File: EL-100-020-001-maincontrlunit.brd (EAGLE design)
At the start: 68 x 86 mm, 13 parts, among them T1 WS-TST-90°, U19 ABS10-32.768KHZ-7-T, U8 MCP7940N-I/SN, U9 PMEG2005ET, X1 944-12-46-00, X2 944-12-46-00

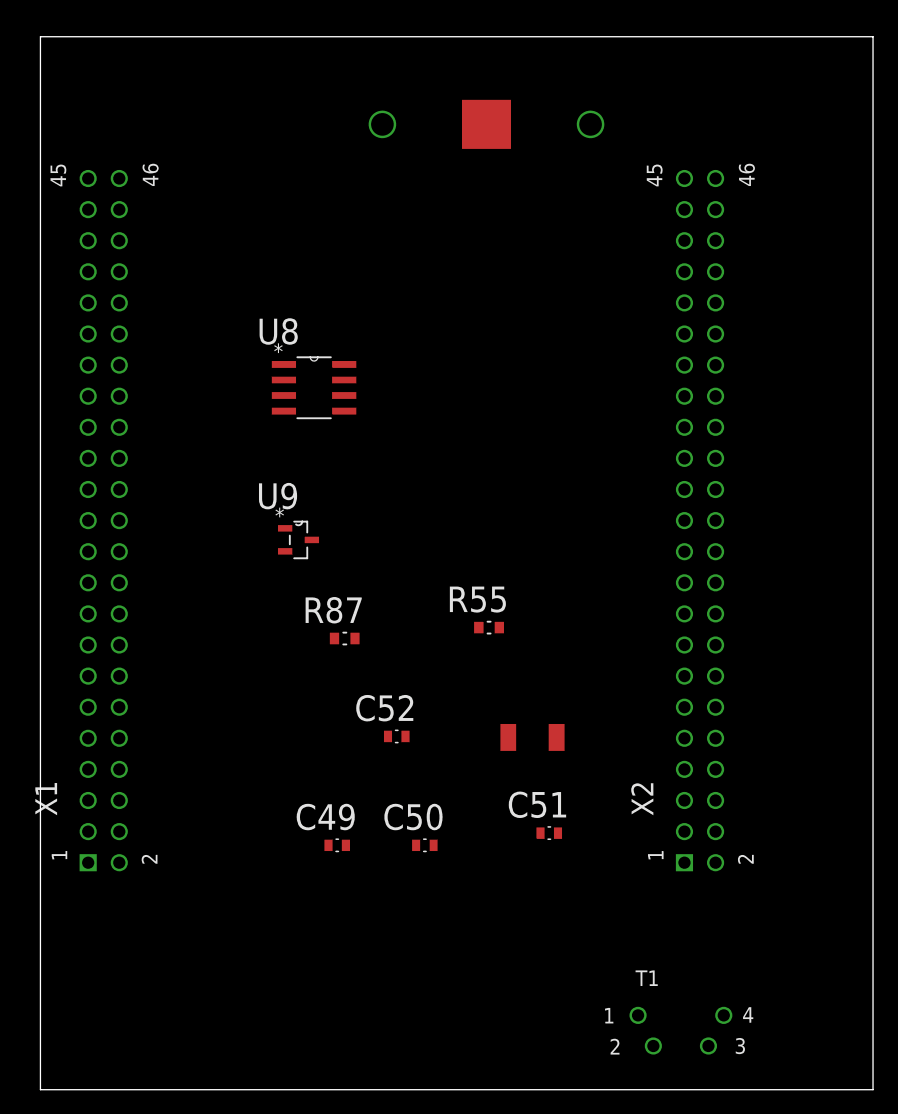
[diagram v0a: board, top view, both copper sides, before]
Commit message: update layout
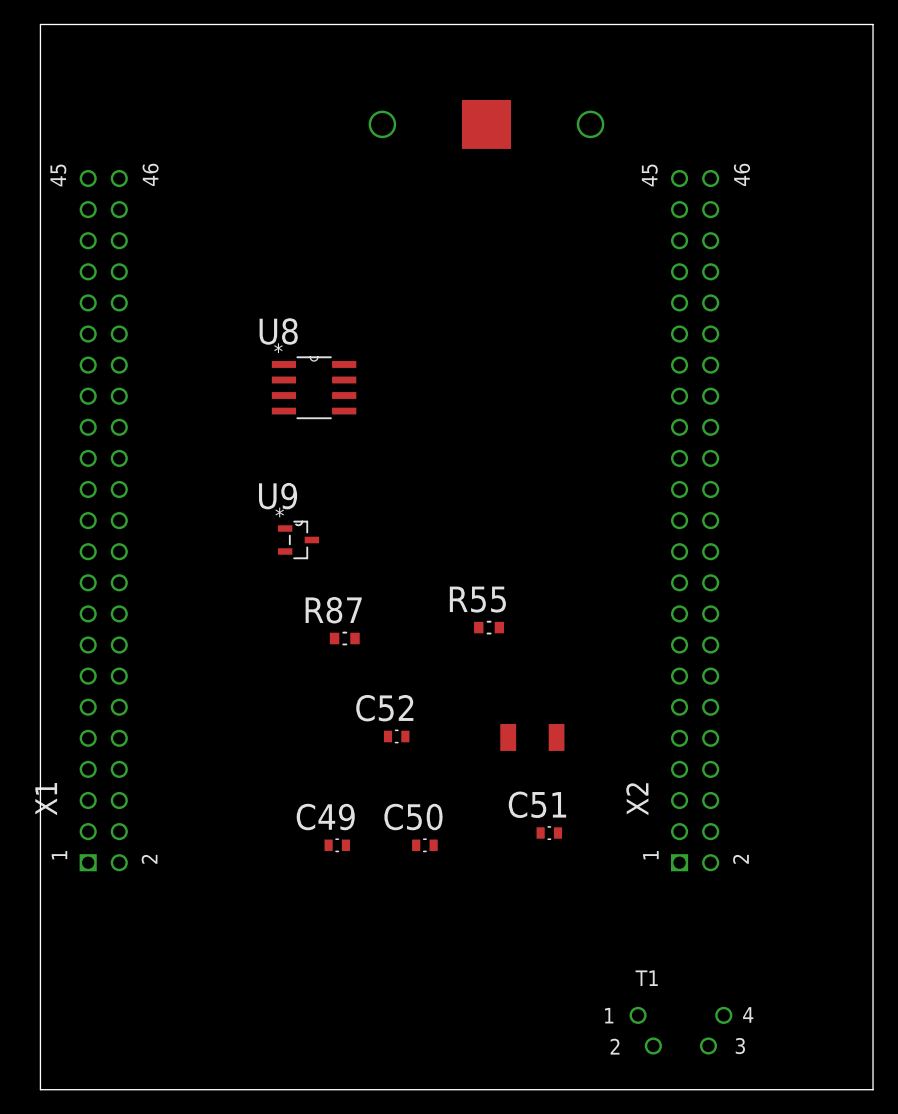
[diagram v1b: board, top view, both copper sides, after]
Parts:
- moved X2 0.40 mm to (52.2, 18.5)
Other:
- board size 68 x 86 mm -> 68 x 87 mm
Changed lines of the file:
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@@
 <setting verticaltext="up"/>
 </settings>
-<grid distance="1" unitdist="mm" unit="mm" style="lines" multiple="1" display="no" altdistance="0.025" altunitdist="inch" altunit="inch"/>
+<grid distance="0.1" unitdist="mm" unit="mm" style="lines" multiple="1" display="no" altdistance="0.025" altunitdist="inch" altunit="inch"/>
 <layers>
 <layer number="1" name="Top" color="4" fill="1" visible="yes" active="yes"/>
-<layer number="2" name="Route2" color="1" fill="3" visible="no" active="yes"/>
+<layer number="2" name="Route2" color="1" fill="3" visible="yes" active="yes"/>
 <layer number="3" name="Route3" color="4" fill="3" visible="no" active="no"/>
 <layer number="14" name="Route14" color="1" fill="6" visible="no" active="no"/>
-<layer number="15" name="Route15" color="4" fill="6" visible="no" active="yes"/>
+<layer number="15" name="Route15" color="4" fill="6" visible="yes" active="yes"/>
 <layer number="16" name="Bottom" color="1" fill="1" visible="yes" active="yes"/>
 <layer number="17" name="Pads" color="2" fill="1" visible="yes" active="yes"/>
@@
 <layer number="45" name="Holes" color="7" fill="1" visible="no" active="yes"/>
 <layer number="46" name="Milling" color="3" fill="1" visible="no" active="yes"/>
-<layer number="47" name="Measures" color="7" fill="1" visible="no" active="yes"/>
+<layer number="47" name="Measures" color="7" fill="1" visible="yes" active="yes"/>
 <layer number="48" name="Document" color="7" fill="1" visible="yes" active="yes"/>
 <layer number="49" name="Reference" color="7" fill="1" visible="yes" active="yes"/>
@@
 <plain>
 <wire x1="0" y1="0" x2="68" y2="0" width="0" layer="20"/>
-<wire x1="68" y1="0" x2="68" y2="86" width="0" layer="20"/>
-<wire x1="68" y1="86" x2="0" y2="86" width="0" layer="20"/>
-<wire x1="0" y1="86" x2="0" y2="0" width="0" layer="20"/>
+<wire x1="68" y1="0" x2="68" y2="87" width="0" layer="20"/>
+<wire x1="68" y1="87" x2="0" y2="87" width="0" layer="20"/>
+<wire x1="0" y1="87" x2="0" y2="0" width="0" layer="20"/>
+<dimension x1="3.9" y1="18.54" x2="52.2" y2="18.54" x3="28.05" y3="11" textsize="1.778" layer="47"/>
+<dimension x1="56" y1="52.8" x2="68" y2="52.8" x3="62" y3="49.6" textsize="1.778" layer="47"/>
 </plain>
 <attributes>
@@
 <attribute name="OC_FARNELL" value="unknown" x="3.9" y="18.54" size="1.778" layer="27" rot="R90" display="off"/>
 </element>
-<element name="X2" library="strasys_standard" package="2,54_STIFTLEIST_2X23" value="944-12-46-00" x="52.6" y="18.54" rot="R90">
-<attribute name="MPN" value="" x="52.6" y="18.54" size="1.778" layer="27" rot="R90" display="off"/>
-<attribute name="SUPPLIER" value="W+P" x="52.6" y="18.54" size="1.778" layer="27" rot="R90" display="off"/>
-<attribute name="MF" value="" x="52.6" y="18.54" size="1.778" layer="27" rot="R90" display="off"/>
-<attribute name="OC_FARNELL" value="unknown" x="52.6" y="18.54" size="1.778" layer="27" rot="R90" display="off"/>
+<element name="X2" library="strasys_standard" package="2,54_STIFTLEIST_2X23" value="944-12-46-00" x="52.2" y="18.54" rot="R90">
+<attribute name="MPN" value="" x="52.2" y="18.54" size="1.778" layer="27" rot="R90" display="off"/>
+<attribute name="SUPPLIER" value="W+P" x="52.2" y="18.54" size="1.778" layer="27" rot="R90" display="off"/>
+<attribute name="MF" value="" x="52.2" y="18.54" size="1.778" layer="27" rot="R90" display="off"/>
+<attribute name="OC_FARNELL" value="unknown" x="52.2" y="18.54" size="1.778" layer="27" rot="R90" display="off"/>
 </element>
 </elements>
@@
 <contactref element="X2" pad="P3"/>
 <contactref element="X2" pad="P4"/>
-<wire x1="52.6" y1="21.08" x2="24.8138" y2="59.235" width="0" layer="19" extent="1-1"/>
-<wire x1="55.14" y1="21.08" x2="52.6" y2="21.08" width="0" layer="19" extent="1-1"/>
-<wire x1="37.4782" y1="37.74" x2="52.6" y2="21.08" width="0" layer="19" extent="1-1"/>
+<wire x1="52.2" y1="21.08" x2="24.8138" y2="59.235" width="0" layer="19" extent="1-1"/>
+<wire x1="54.74" y1="21.08" x2="52.2" y2="21.08" width="0" layer="19" extent="1-1"/>
+<wire x1="37.4782" y1="37.74" x2="52.2" y2="21.08" width="0" layer="19" extent="1-1"/>
 <wire x1="24.9512" y1="19.96" x2="37.4782" y2="37.74" width="0" layer="19" extent="1-1"/>
 </signal>
@@
 <contactref element="X2" pad="P44"/>
 <contactref element="X2" pad="P46"/>
-<wire x1="55.14" y1="74.42" x2="36.43" y2="78.84" width="0" layer="19" extent="1-1"/>
-<wire x1="52.6" y1="74.42" x2="55.14" y2="74.42" width="0" layer="19" extent="1-1"/>
-<wire x1="55.14" y1="71.88" x2="55.14" y2="74.42" width="0" layer="19" extent="1-1"/>
-<wire x1="52.6" y1="71.88" x2="52.6" y2="74.42" width="0" layer="19" extent="1-1"/>
-<wire x1="19.8862" y1="55.425" x2="52.6" y2="71.88" width="0" layer="19" extent="1-1"/>
+<wire x1="54.74" y1="74.42" x2="36.43" y2="78.84" width="0" layer="19" extent="1-1"/>
+<wire x1="52.2" y1="74.42" x2="54.74" y2="74.42" width="0" layer="19" extent="1-1"/>
+<wire x1="54.74" y1="71.88" x2="54.74" y2="74.42" width="0" layer="19" extent="1-1"/>
+<wire x1="52.2" y1="71.88" x2="52.2" y2="74.42" width="0" layer="19" extent="1-1"/>
+<wire x1="19.8862" y1="55.425" x2="52.2" y2="71.88" width="0" layer="19" extent="1-1"/>
 <wire x1="6.44" y1="18.54" x2="19.8862" y2="55.425" width="0" layer="19" extent="1-1"/>
 <wire x1="3.9" y1="18.54" x2="6.44" y2="18.54" width="0" layer="19" extent="1-1"/>
-<wire x1="52.6" y1="18.54" x2="6.44" y2="18.54" width="0" layer="19" extent="1-1"/>
-<wire x1="55.14" y1="18.54" x2="52.6" y2="18.54" width="0" layer="19" extent="1-1"/>
-<wire x1="54.56" y1="3.57" x2="55.14" y2="18.54" width="0" layer="19" extent="1-1"/>
+<wire x1="52.2" y1="18.54" x2="6.44" y2="18.54" width="0" layer="19" extent="1-1"/>
+<wire x1="54.74" y1="18.54" x2="52.2" y2="18.54" width="0" layer="19" extent="1-1"/>
+<wire x1="54.56" y1="3.57" x2="54.74" y2="18.54" width="0" layer="19" extent="1-1"/>
 <wire x1="28.3888" y1="28.85" x2="54.56" y2="3.57" width="0" layer="19" extent="1-1"/>
 <wire x1="40.8488" y1="20.96" x2="28.3888" y2="28.85" width="0" layer="19" extent="1-1"/>
@@
 <contactref element="U8" pad="5"/>
 <contactref element="X2" pad="P18"/>
-<wire x1="24.8138" y1="55.425" x2="55.14" y2="38.86" width="0" layer="19" extent="1-1"/>
+<wire x1="24.8138" y1="55.425" x2="54.74" y2="38.86" width="0" layer="19" extent="1-1"/>
 </signal>
 <signal name="I2C1_SCL">
 <contactref element="U8" pad="6"/>
 <contactref element="X2" pad="P17"/>
-<wire x1="24.8138" y1="56.695" x2="52.6" y2="38.86" width="0" layer="19" extent="1-1"/>
+<wire x1="24.8138" y1="56.695" x2="52.2" y2="38.86" width="0" layer="19" extent="1-1"/>
 </signal>
 <signal name="SYS_RESET">
 <contactref element="T1" pad="2"/>
 <contactref element="X2" pad="P10"/>
-<wire x1="50.06" y1="3.57" x2="55.14" y2="28.7" width="0" layer="19" extent="1-1"/>
+<wire x1="50.06" y1="3.57" x2="54.74" y2="28.7" width="0" layer="19" extent="1-1"/>
 </signal>
 <signal name="PE">
@@
 <contactref element="X2" pad="P6"/>
 <contactref element="X2" pad="P5"/>
-<wire x1="52.6" y1="23.62" x2="55.14" y2="23.62" width="0" layer="19" extent="1-1"/>
+<wire x1="52.2" y1="23.62" x2="54.74" y2="23.62" width="0" layer="19" extent="1-1"/>
 </signal>
 <signal name="SYS5V">
 <contactref element="X2" pad="P7"/>
 <contactref element="X2" pad="P8"/>
-<wire x1="52.6" y1="26.16" x2="55.14" y2="26.16" width="0" layer="19" extent="1-1"/>
+<wire x1="52.2" y1="26.16" x2="54.74" y2="26.16" width="0" layer="19" extent="1-1"/>
 </signal>
 <signal name="PWR_BUT">
